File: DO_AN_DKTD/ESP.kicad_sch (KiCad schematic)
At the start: 11 parts, among them J4 , SW2 SW_Push, SW3 SW_Push, U10 ESP-07

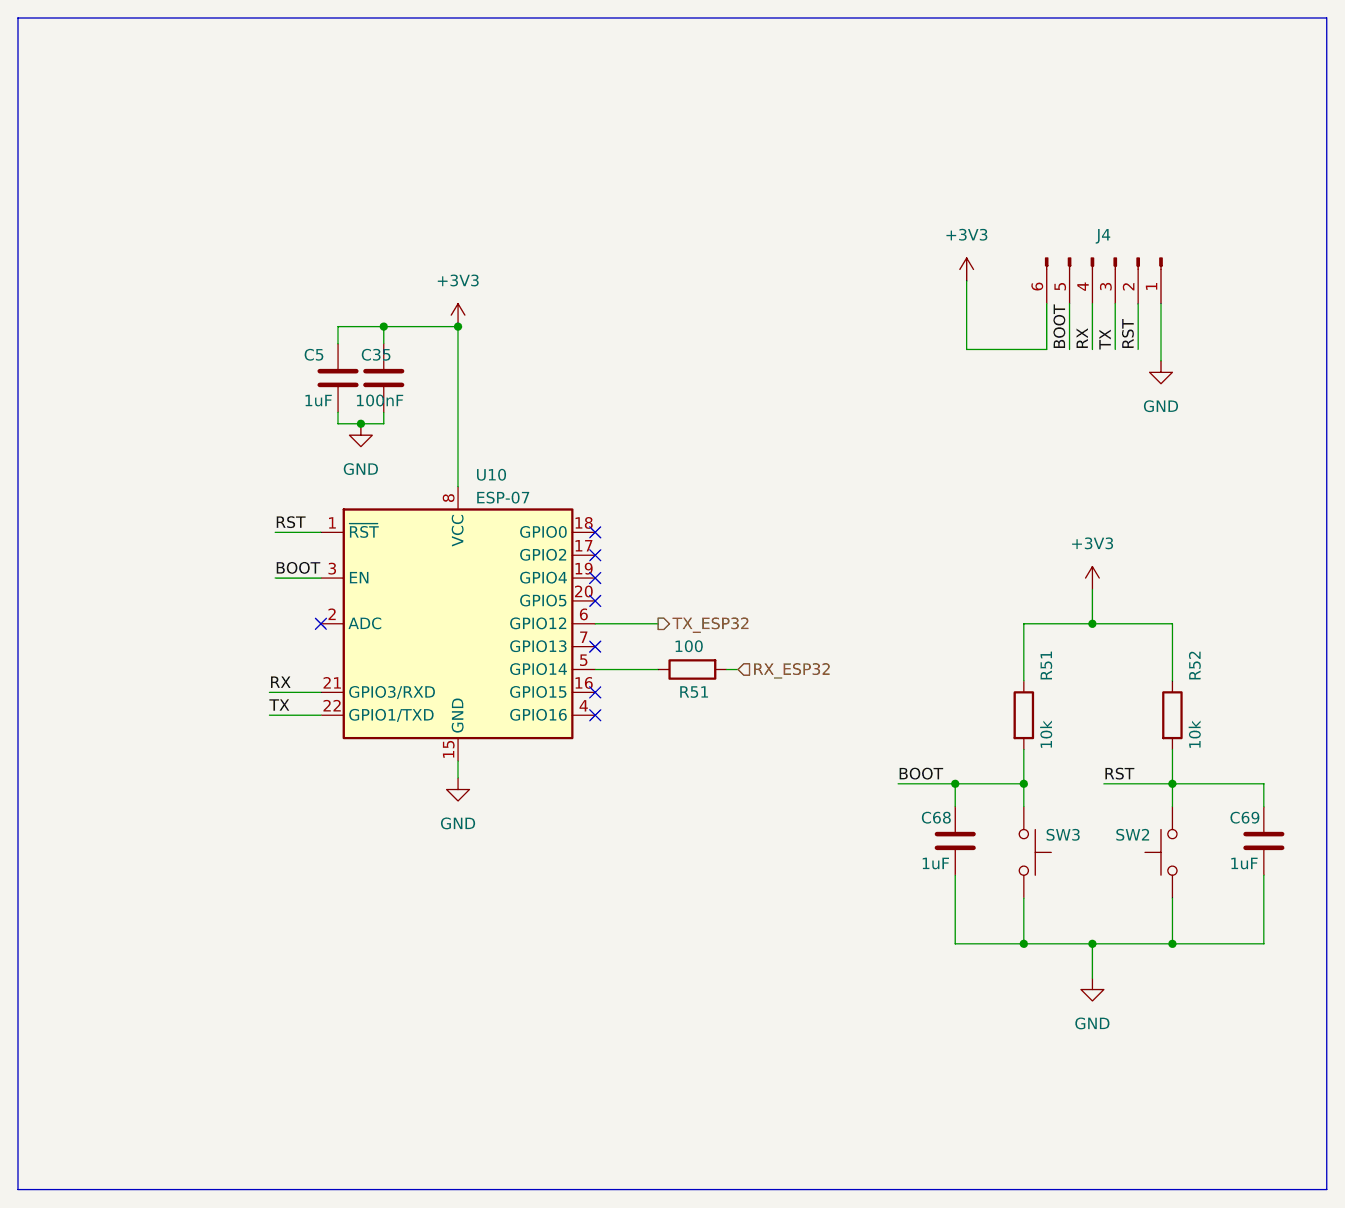
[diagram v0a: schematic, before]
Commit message: commit to change branch
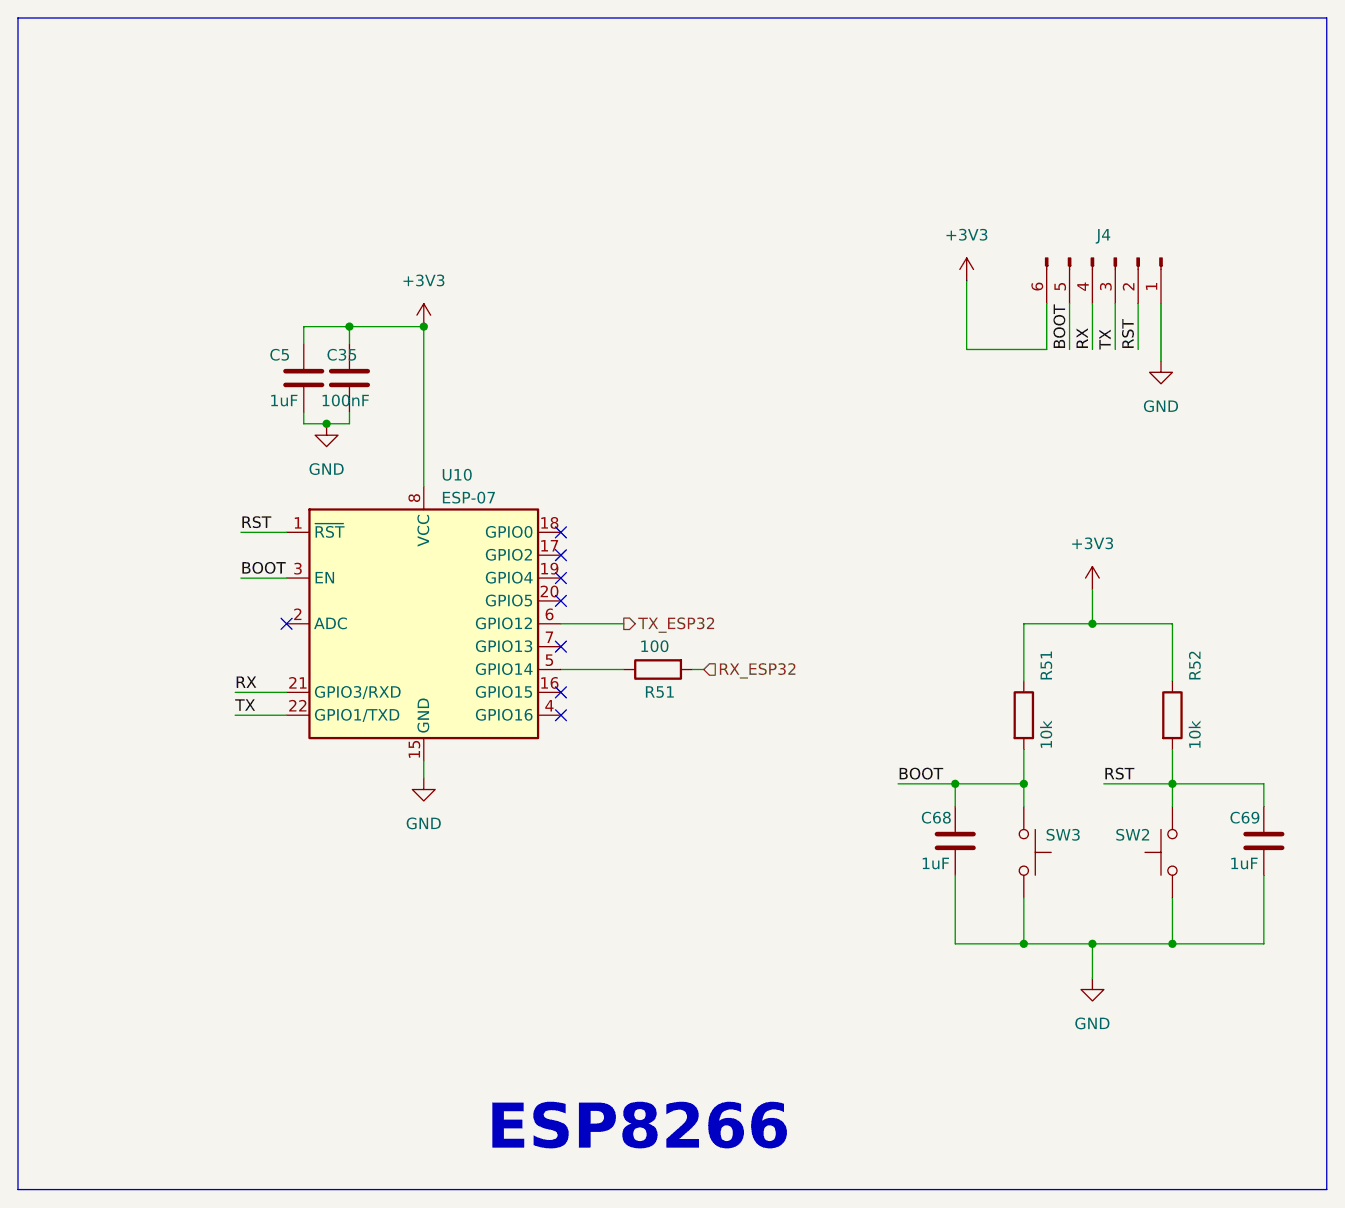
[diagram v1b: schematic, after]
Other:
- note added: "ESP8266"
- moved on the sheet: C35, C5, R51, U10
